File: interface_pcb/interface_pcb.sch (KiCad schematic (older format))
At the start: 6 parts

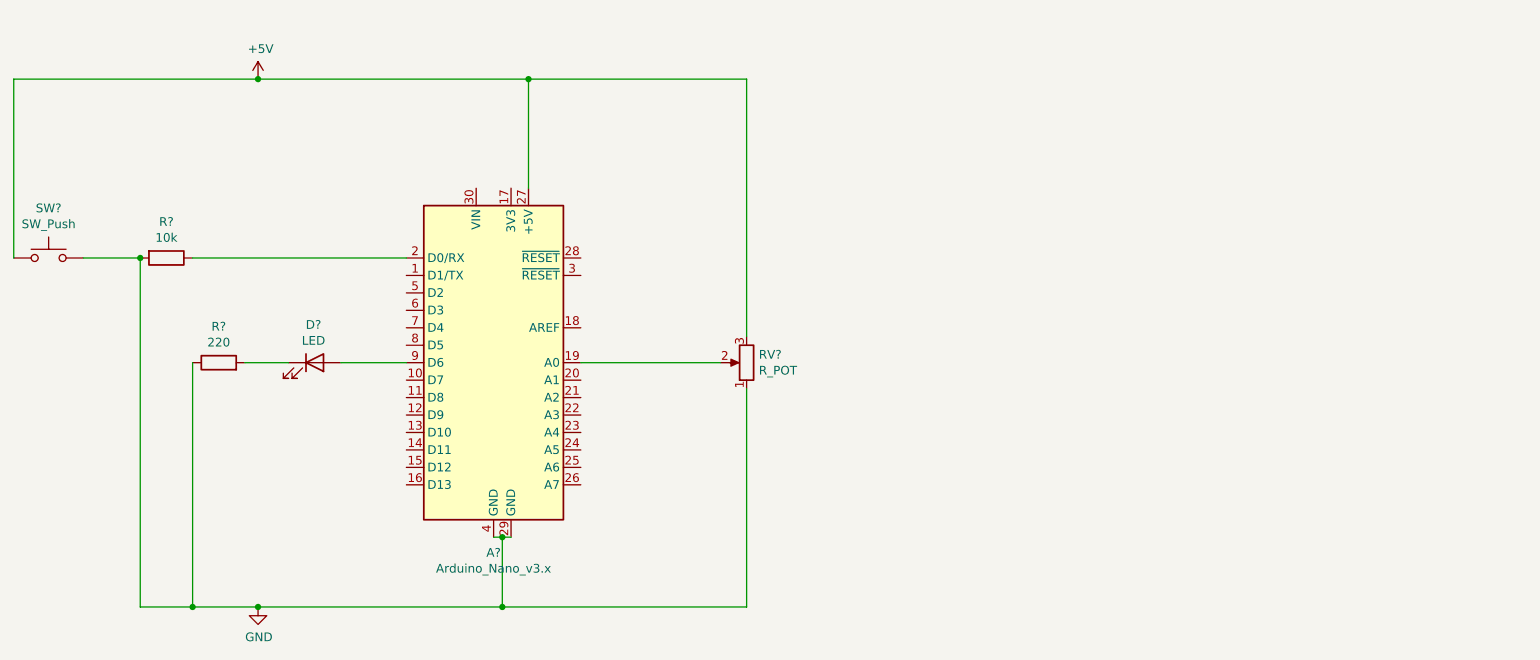
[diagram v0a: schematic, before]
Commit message: Add 4 of each
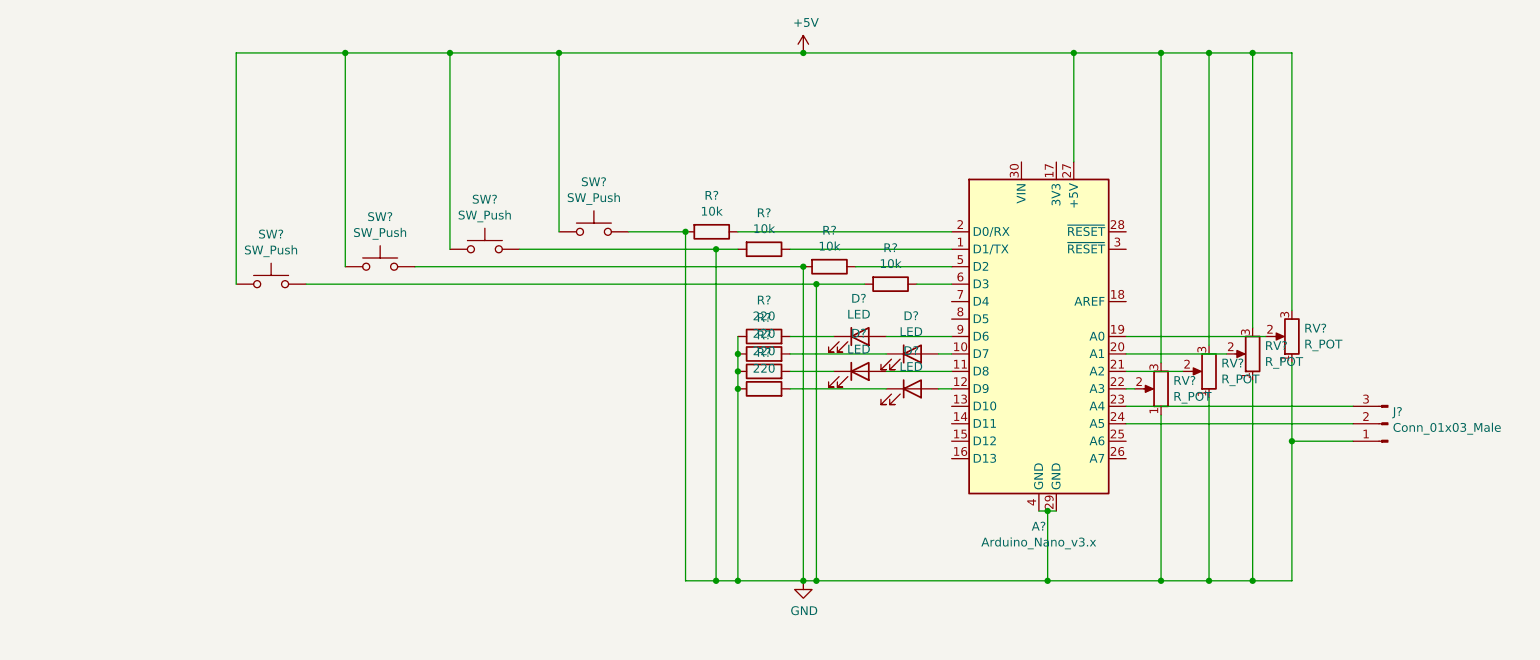
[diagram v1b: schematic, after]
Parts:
- added D? (x3): LED, symbol Device:LED
- added J?: Conn_01x03_Male, symbol Connector:Conn_01x03_Male
- added R? (x3): 10k, symbol Device:R
- added R? (x3): 220, symbol Device:R
- added RV? (x3): R_POT, symbol Device:R_POT
- added SW? (x3): SW_Push, symbol Switch:SW_Push
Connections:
- net +5V: now also RV?.3, RV?.3, RV?.3, SW?.1, SW?.1, SW?.1
- net GND: now also J?.1 (Pin_1), R?.1, R?.1, R?.1, R?.2, R?.2, R?.2, RV?.1, RV?.1, RV?.1, SW?.2, SW?.2, SW?.2
- net at A?.1 (D1/TX): now also R?.1
- net at A?.10 (D7): now also D?.2 (A)
- net at A?.11 (D8): now also D?.2 (A)
- net at A?.12 (D9): now also D?.2 (A)
- net at A?.20 (A1): now also RV?.2
- net at A?.21 (A2): now also RV?.2
- net at A?.22 (A3): now also RV?.2
- net at A?.23 (A4): now also J?.3 (Pin_3)
- net at A?.24 (A5): now also J?.2 (Pin_2)
- net at A?.5 (D2): now also R?.1
- net at A?.6 (D3): now also R?.1
- new net: D?.1 (K), R?.2 (x3)
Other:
- moved on the sheet: A?, D?, R?, RV?, SW?
